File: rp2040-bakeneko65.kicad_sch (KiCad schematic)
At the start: 31 parts, among them J1 SM04B-SRSS-TB, J2 SWD, SW85 SW_Push, U1 RP2040, U2 W25Q128JVS, U3 XC6206PxxxMR, U4 SRV05-4, Y1 12MHz

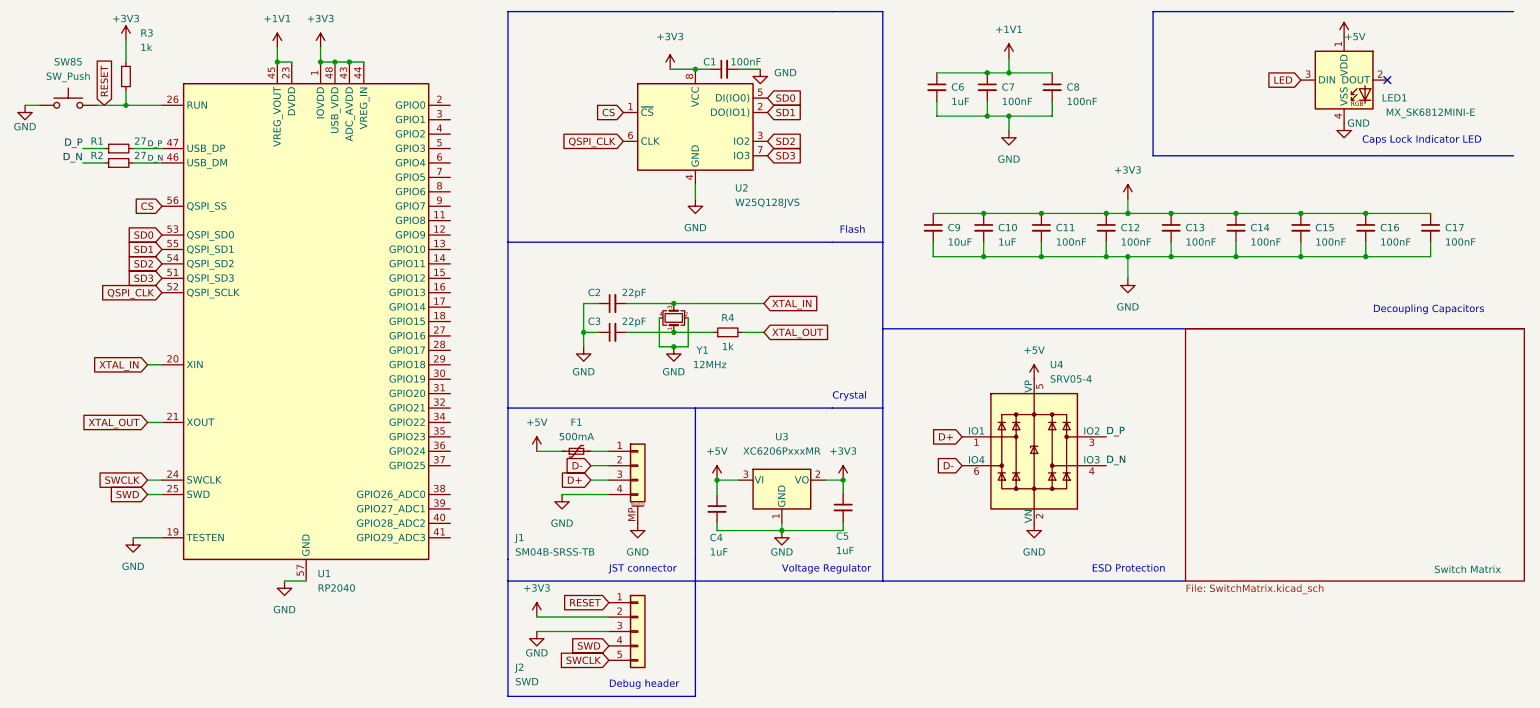
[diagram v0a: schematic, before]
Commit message: flash, redo ESD, some other stuff
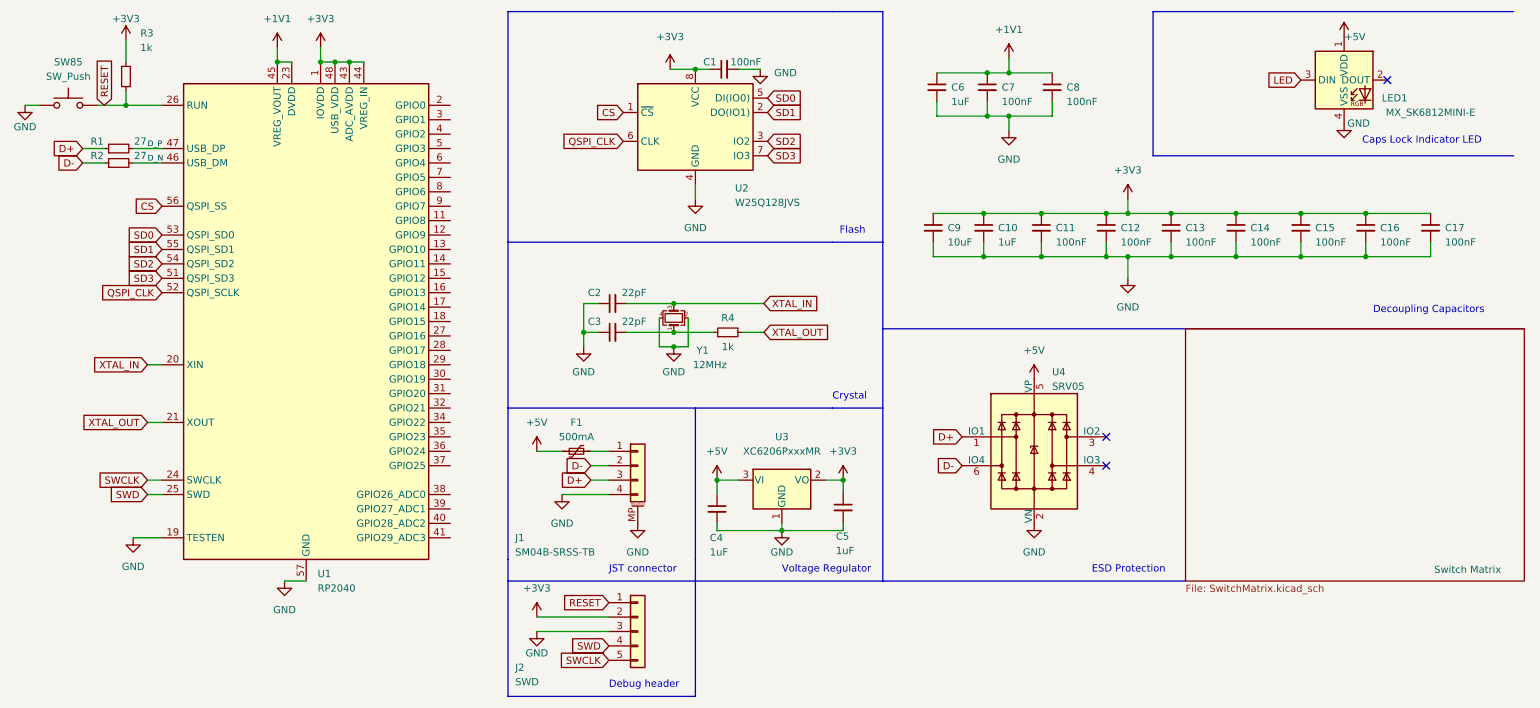
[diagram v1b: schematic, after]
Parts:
- U4: value SRV05-4 -> SRV05
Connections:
- net D+: now also R1.1
- net D-: now also R2.1
- net D_N: no longer R2.1, U4.4 (IO3)
- net D_P: no longer R1.1, U4.3 (IO2)
- no-connect marks 1 -> 3
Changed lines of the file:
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@@
   )
   (no_connect (at 262.89 24.765))
+  (no_connect (at 213.36 87.63))
+  (no_connect (at 213.36 92.71))
   (wire (pts (xy 74.93 21.59) (xy 77.47 21.59))
     (stroke (width 0) (type default))
@@
   (label "D_N" (at 44.45 39.37 0) (fields_autoplaced)
     (effects (font (size 1 1)) (justify left bottom))
-  )
-  (label "D_N" (at 213.36 92.71 0) (fields_autoplaced)
-    (effects (font (size 1.27 1.27)) (justify left bottom))
-  )
-  (label "D_P" (at 33.02 36.83 180) (fields_autoplaced)
-    (effects (font (size 1.27 1.27)) (justify right bottom))
-  )
-  (label "D_P" (at 213.36 87.63 0) (fields_autoplaced)
-    (effects (font (size 1.27 1.27)) (justify left bottom))
-  )
-  (label "D_N" (at 33.02 39.37 180) (fields_autoplaced)
-    (effects (font (size 1.27 1.27)) (justify right bottom))
   )
   (global_label "XTAL_OUT" (shape input) (at 44.45 85.09 180) (fields_autoplaced)
@@
     )
   )
+  (global_label "D+" (shape input) (at 33.02 36.83 180) (fields_autoplaced)
+    (effects (font (size 1.27 1.27)) (justify right))
+    (property "Intersheetrefs" "${INTERSHEET_REFS}" (at 27.2718 36.83 0)
+      (effects (font (size 1.27 1.27)) (justify right) hide)
+    )
+  )
   (global_label "CS" (shape input) (at 46.99 46.99 180) (fields_autoplaced)
     (effects (font (size 1.27 1.27)) (justify right))
@@
     )
   )
+  (global_label "D-" (shape input) (at 33.02 39.37 180) (fields_autoplaced)
+    (effects (font (size 1.27 1.27)) (justify right))
+    (property "Intersheetrefs" "${INTERSHEET_REFS}" (at 27.2718 39.37 0)
+      (effects (font (size 1.27 1.27)) (justify right) hide)
+    )
+  )
   (global_label "QSPI_CLK" (shape input) (at 128.27 35.56 180) (fields_autoplaced)
     (effects (font (size 1.27 1.27)) (justify right))
@@
   (symbol (lib_id "marbastlib-various:SRV05-4") (at 200.66 90.17 0) (unit 1)
     (in_bom yes) (on_board yes) (dnp no) (fields_autoplaced)
-    (property "Reference" "U4" (at 203.4287 74.93 0)
+    (property "Reference" "U4" (at 203.8097 76.2 0)
       (effects (font (size 1.27 1.27)) (justify left))
     )
-    (property "Value" "SRV05-4" (at 203.4287 77.47 0)
+    (property "Value" "SRV05" (at 203.8097 78.74 0)
       (effects (font (size 1.27 1.27)) (justify left))
     )

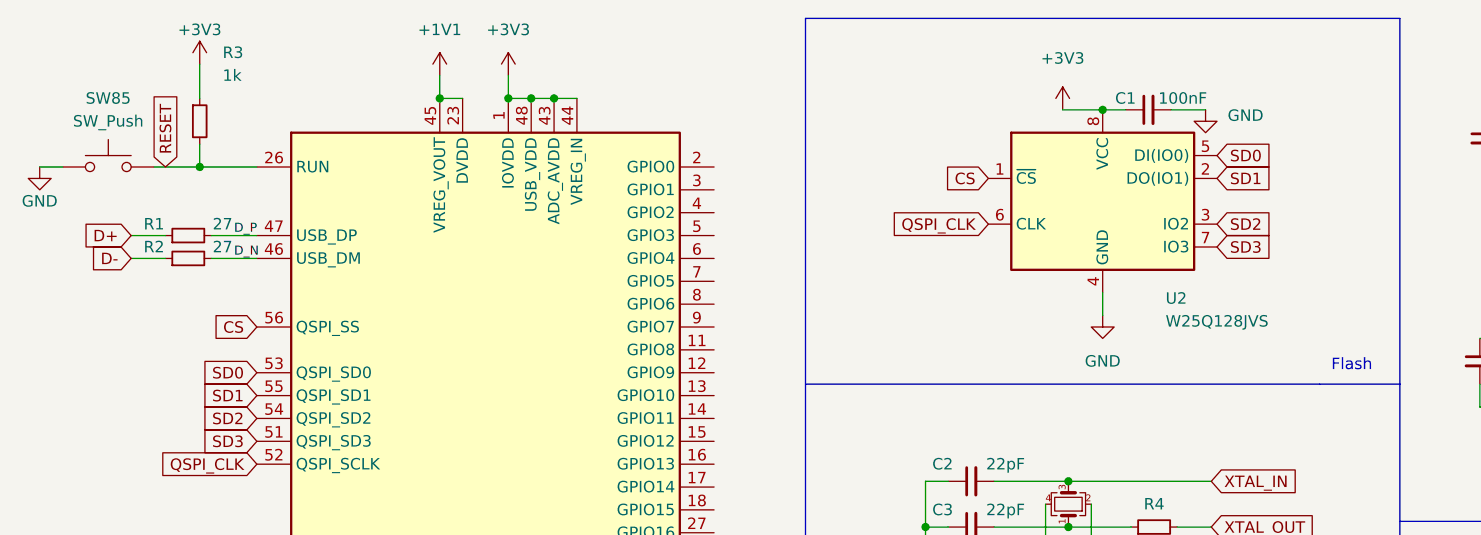
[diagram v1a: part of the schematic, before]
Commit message: USB boot
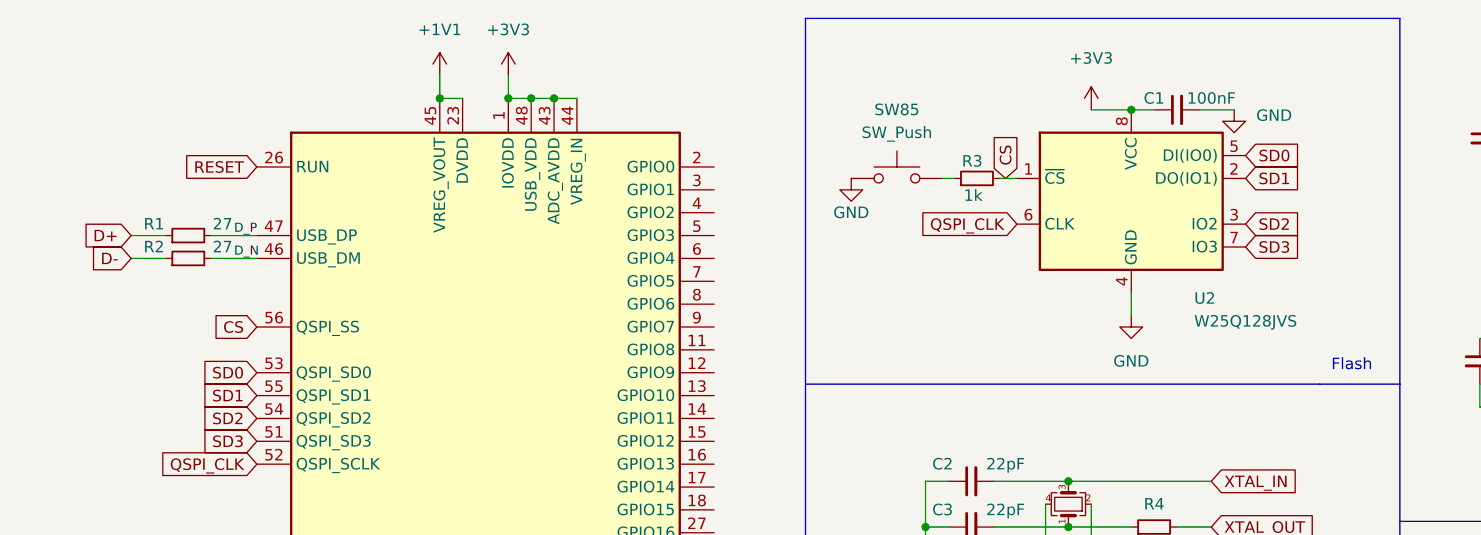
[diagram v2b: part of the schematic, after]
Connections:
- net +3V3: no longer R3.1
- net CS: now also R3.2
- net RESET: no longer R3.2, SW85.2
- new net: R3.1, SW85.2
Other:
- moved on the sheet: C1, R3, SW85, U2
